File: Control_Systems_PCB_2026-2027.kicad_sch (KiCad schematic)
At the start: 11 parts, among them U1 STM32F446VETx

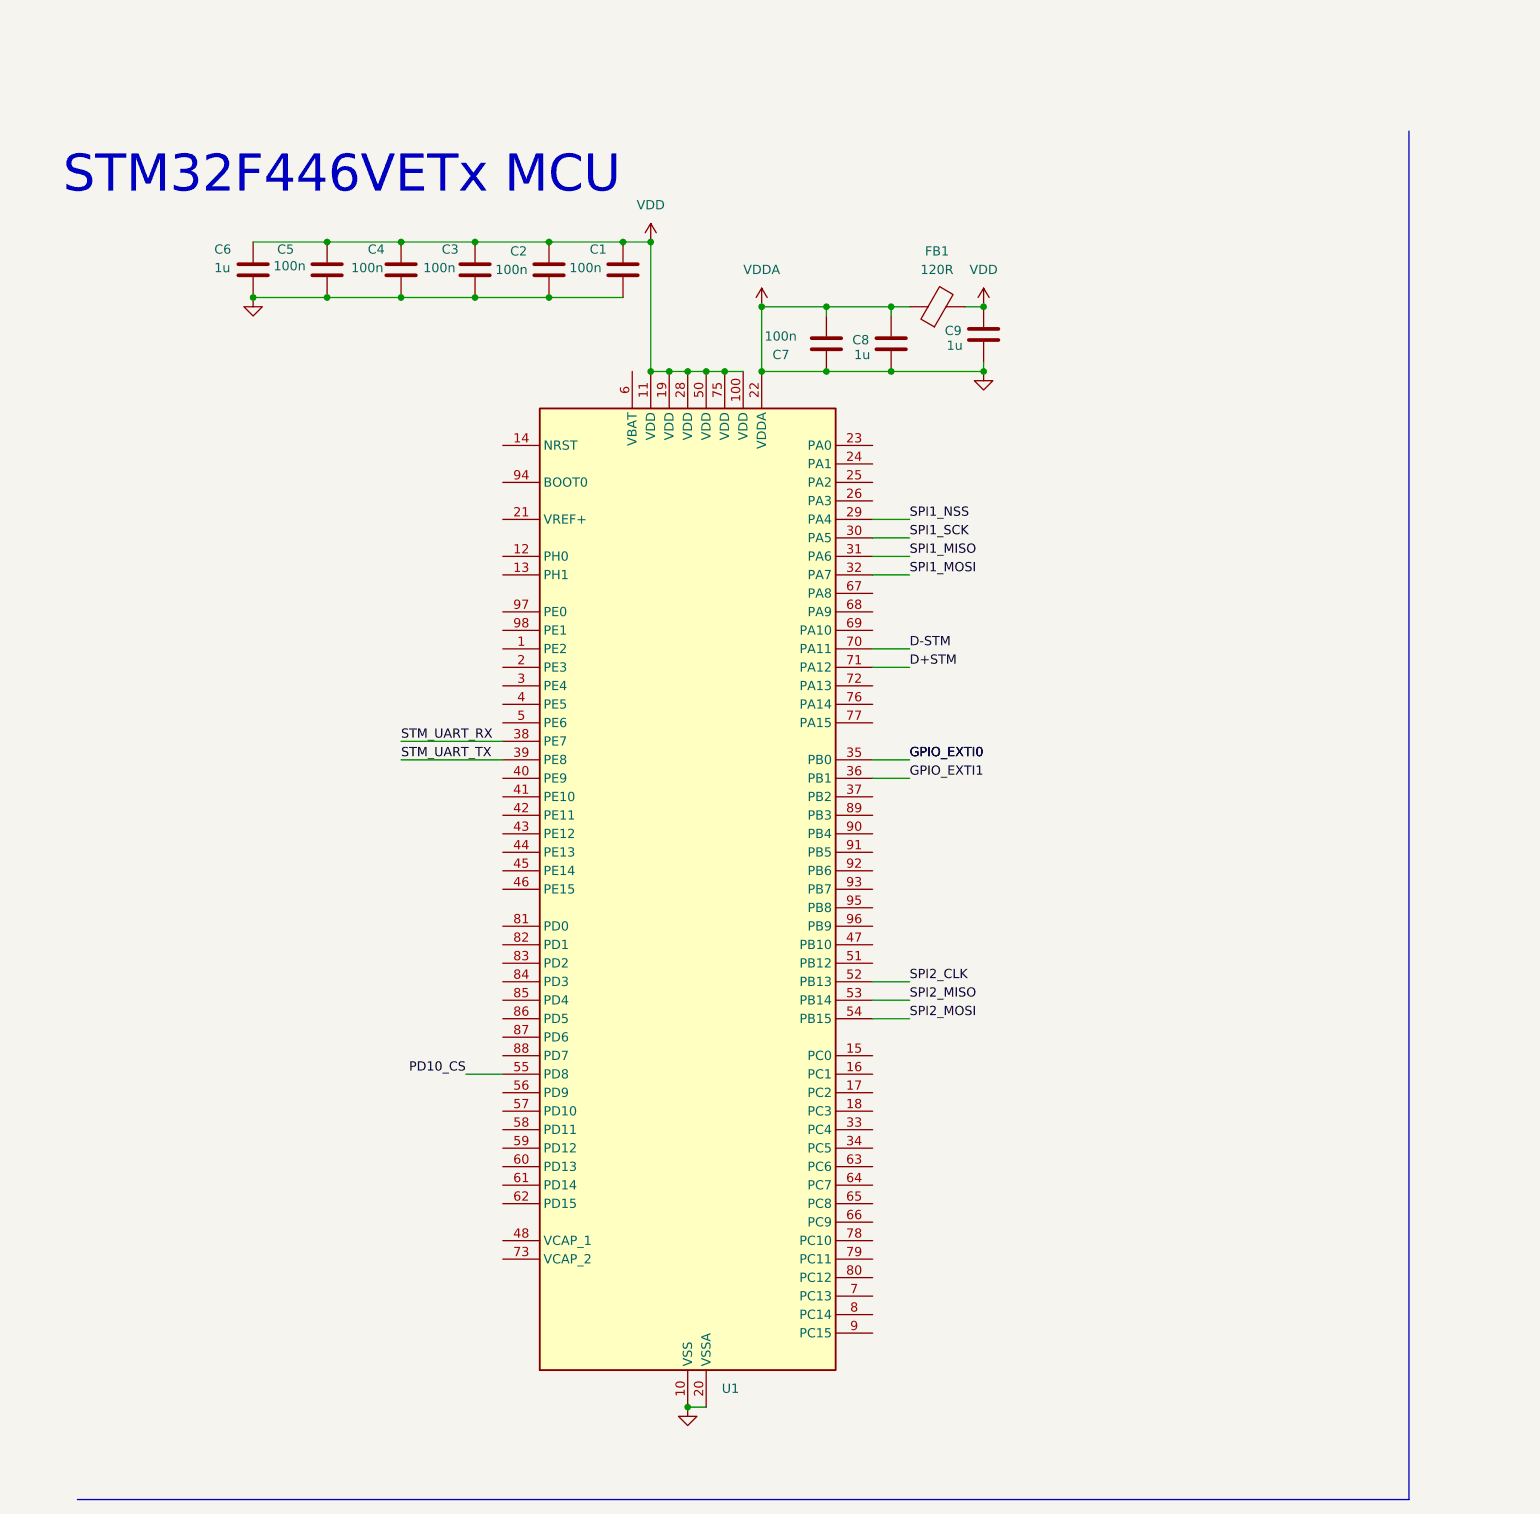
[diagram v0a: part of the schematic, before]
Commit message: fahhh
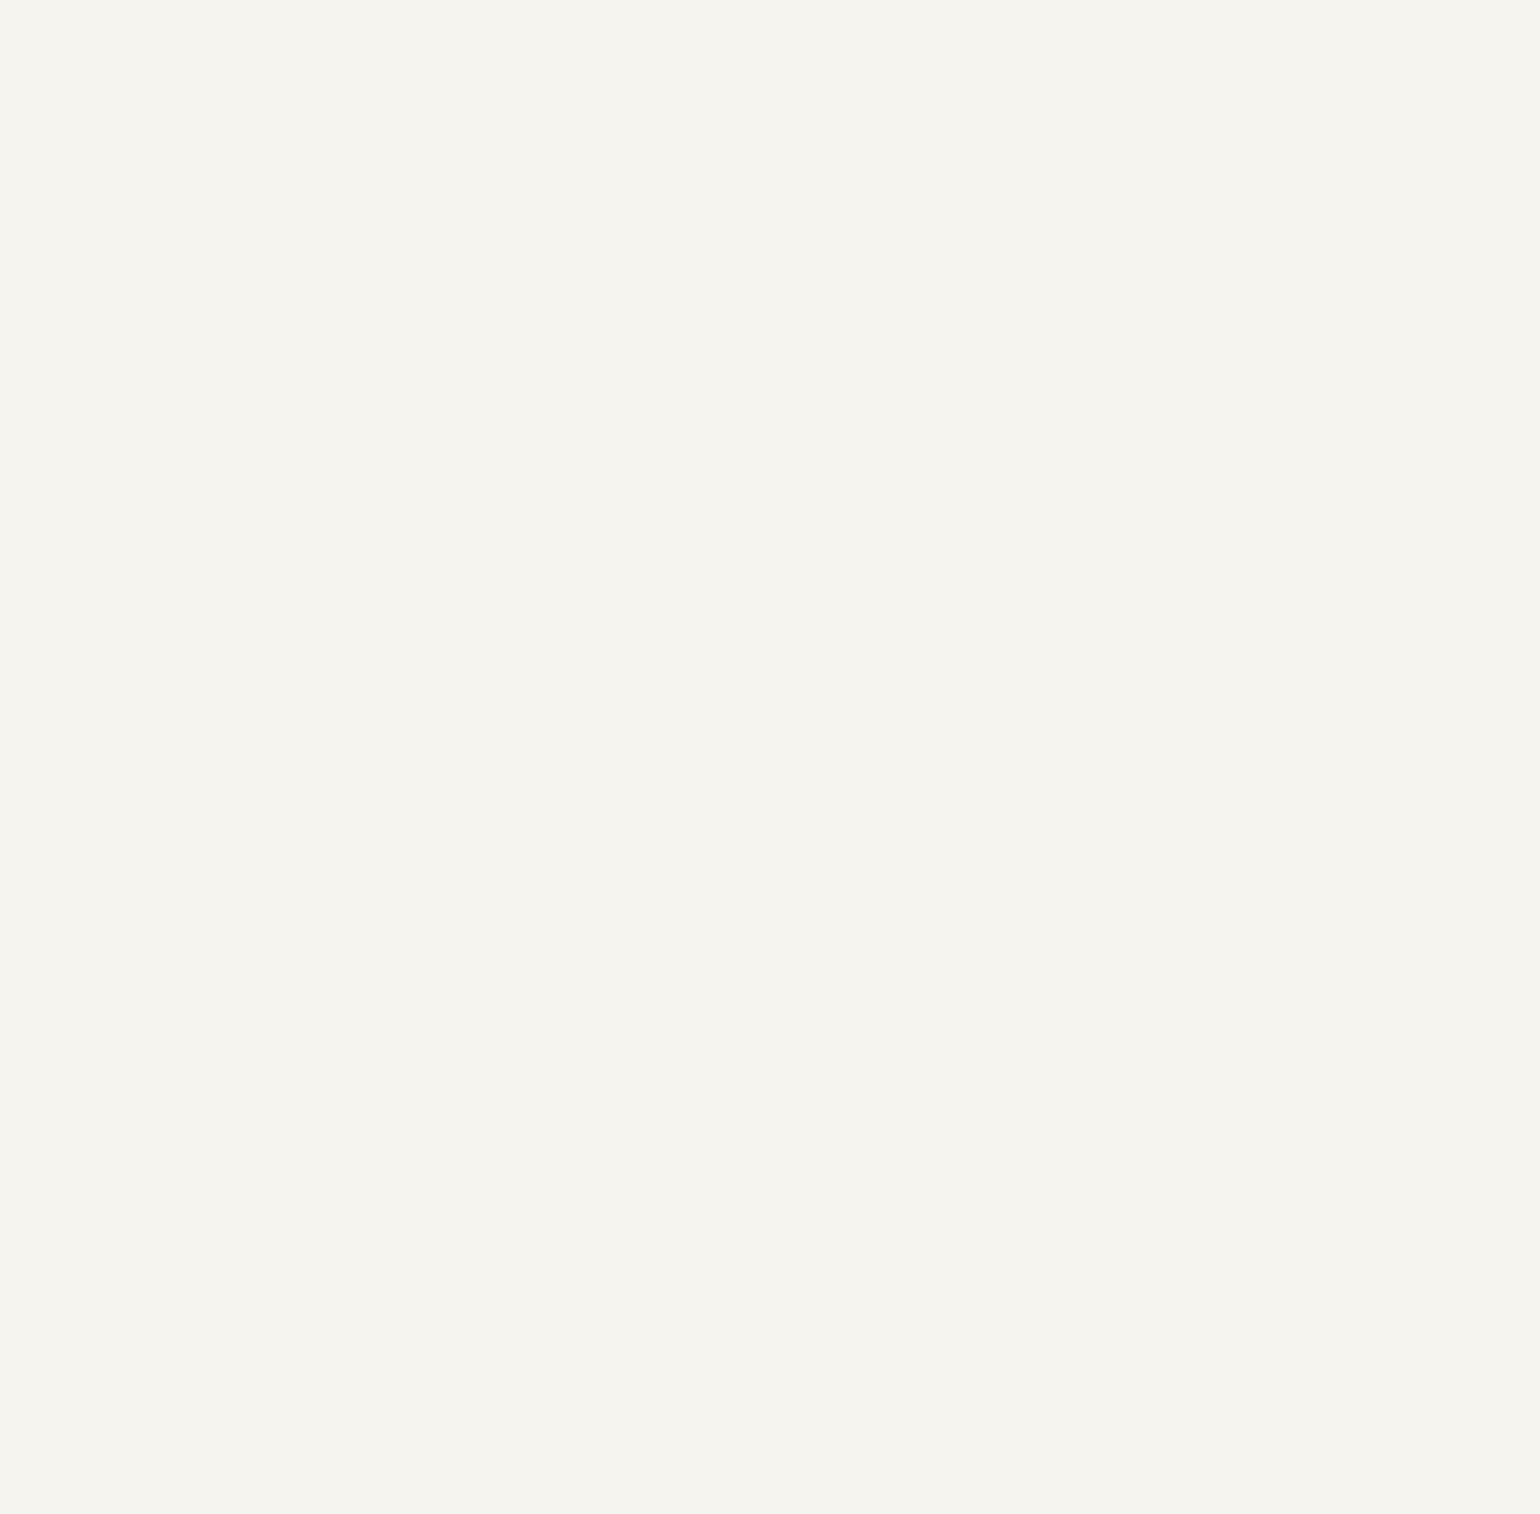
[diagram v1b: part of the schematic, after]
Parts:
- removed C1, C2, C3, C4, C5, C7: 100n, symbol Device:C
- removed C6, C8, C9: 1u, symbol Device:C
- removed FB1: 120R, symbol Device:FerriteBead
- removed U1: STM32F446VETx, Package_QFP:LQFP-100_14x14mm_P0.5mm, symbol MCU_ST_STM32F4:STM32F446VETx
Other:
- note removed: "STM32F446VETx MCU"
